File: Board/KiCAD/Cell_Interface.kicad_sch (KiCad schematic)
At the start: 26 parts, among them Q23 2N7002, Q24 2N7002, Q25 2N7002, Q26 2N7002, Q5 BSS83P, Q6 BSS83P, Q7 BSS83P, Q8 BSS83P, U6 INA219AxDCN, U7 INA219AxDCN, U8 INA219AxDCN

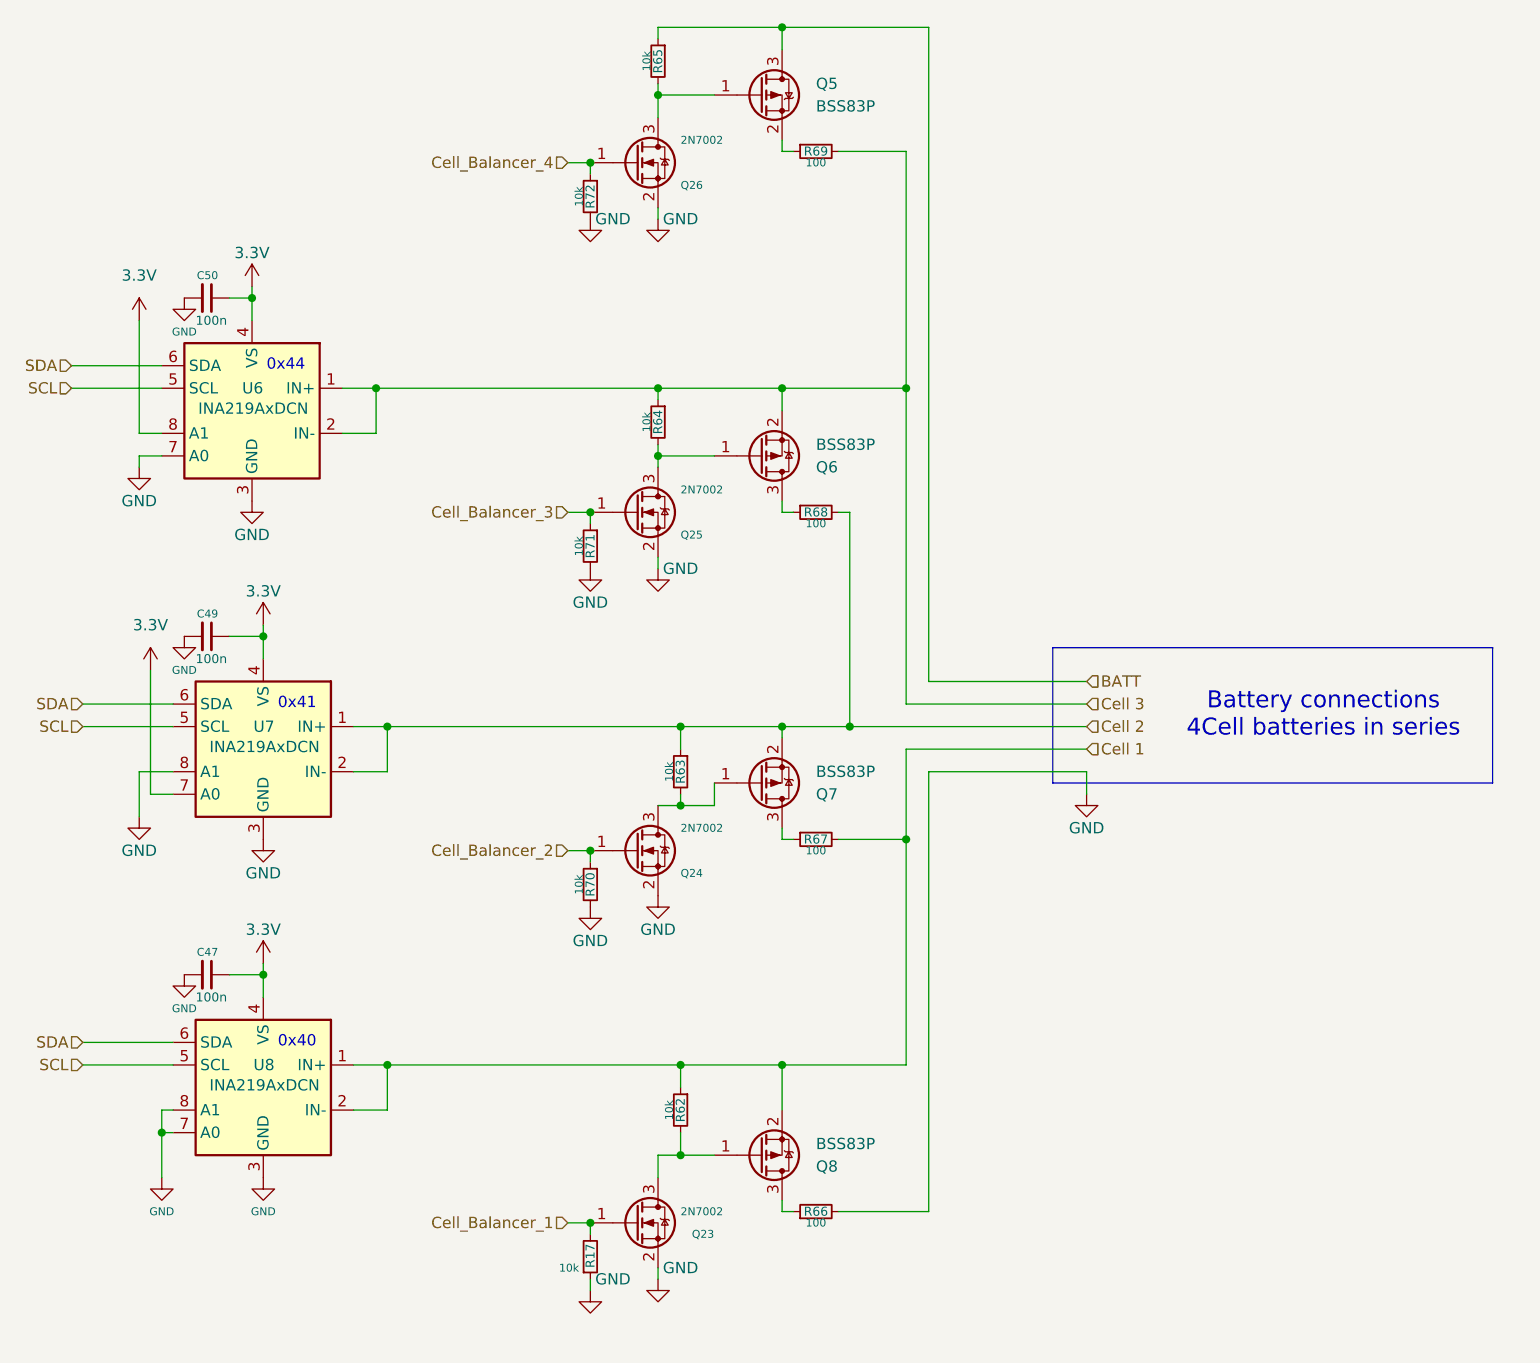
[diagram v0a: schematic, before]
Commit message: BOM Complete Need a Once Over Check
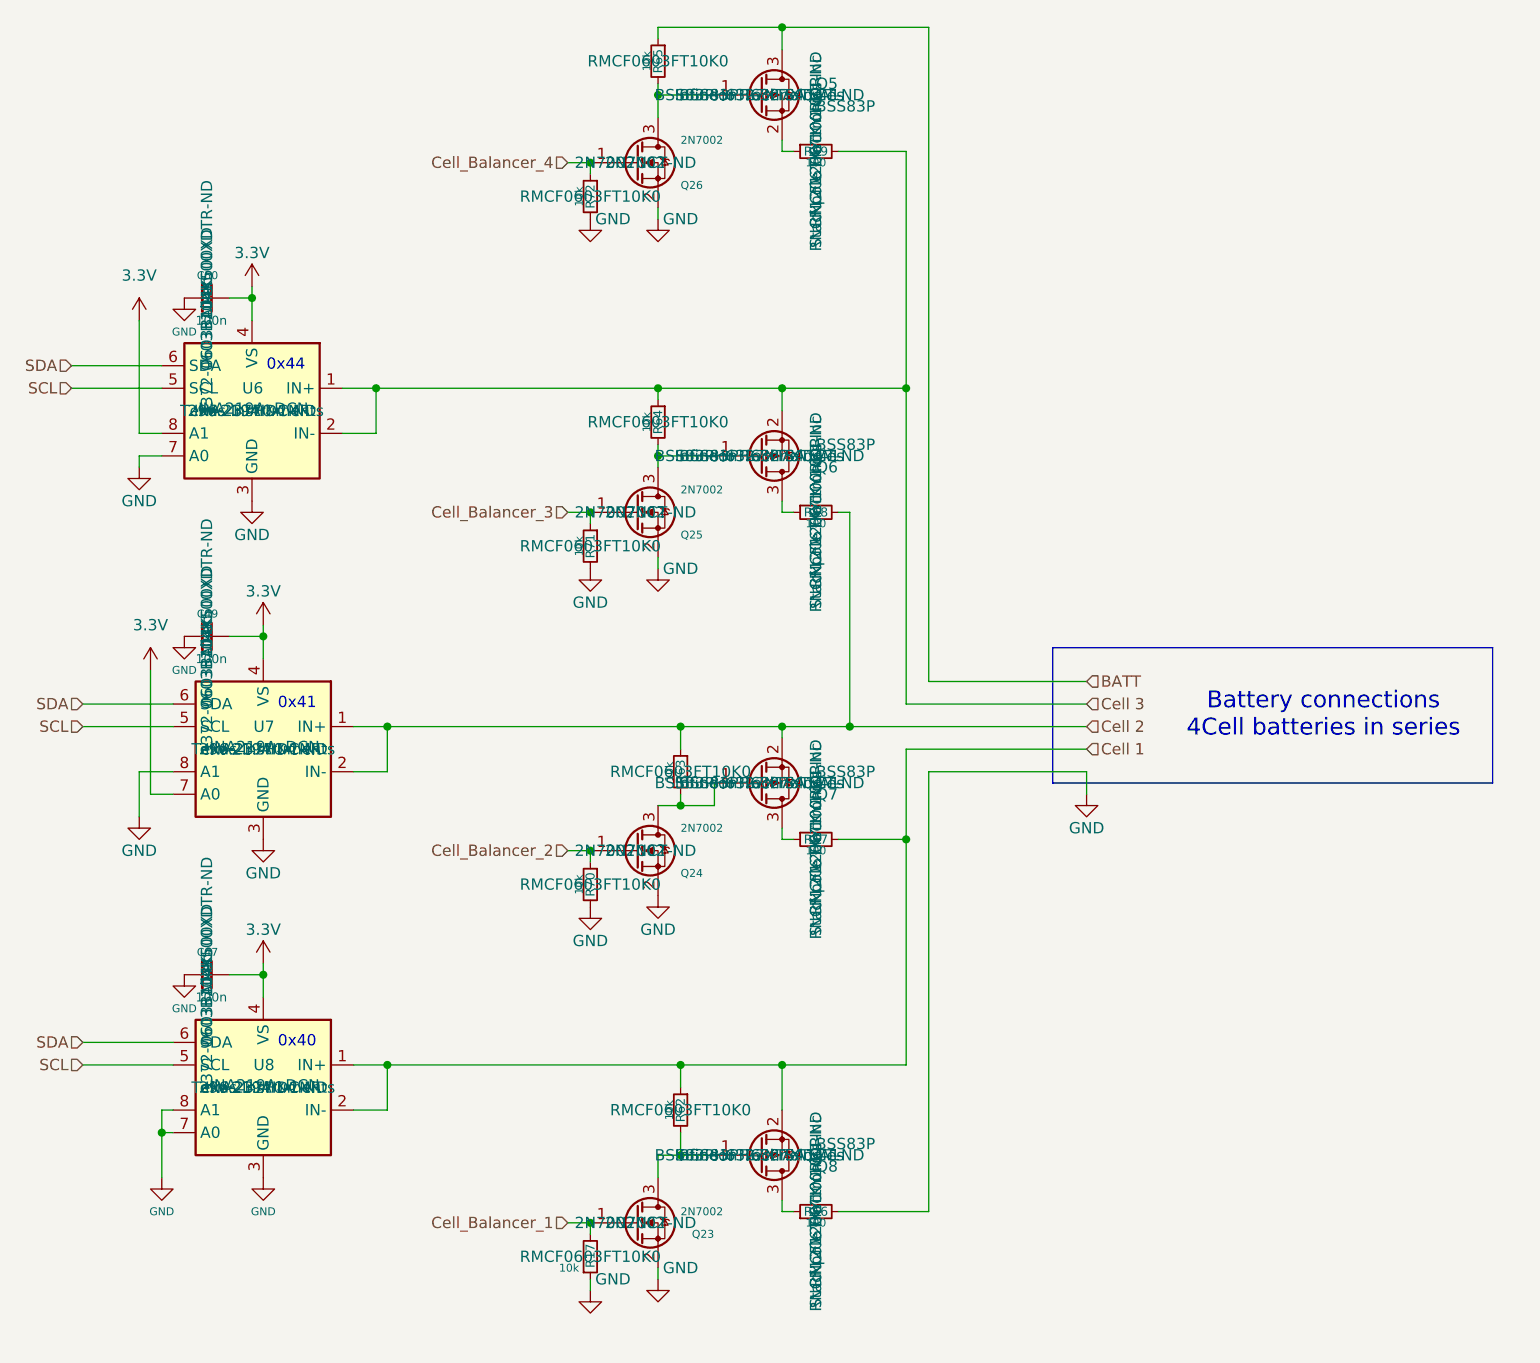
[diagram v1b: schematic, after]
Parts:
- C47, C49, C50: MFR (none) -> Aillen; MPN (none) -> 3372-0603B104K500XDTR-ND; Package (none) -> 0603B104K500XD
- Q23, Q24, Q25, Q26: MFR Alpha & Omega Semiconductor -> onsemi; MPN (none) -> 2N7002NCT-ND; Package (none) -> 2N7002
- Q5, Q6, Q7, Q8: MFR (none) -> Infineon Technologies; MPN (none) -> BSS83PH6327XTSA1CT-ND; Package (none) -> BSS83PH6327XTSA1
- R17, R62, R63, R64, R65, R70, R71, R72: MPN RMCF0603FT10K0 -> RMCF0603FT10K0CT-ND; Package (none) -> RMCF0603FT10K0
- R66, R67, R68, R69: MFR (none) -> Stackpole Electronics Inc; MPN (none) -> RNCF1206TKY100RCT-ND; Package (none) -> RNCF1206TKY100R
- U6, U7, U8: MFR (none) -> Texas Instruments; MPN (none) -> 296-23770-1-ND; Package (none) -> INA219AIDCNR
